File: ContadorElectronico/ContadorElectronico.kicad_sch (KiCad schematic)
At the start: 27 parts, among them J1 Screw_Terminal_01x02, J2 Screw_Terminal_01x02, SW1 MODE, SW2 INC, SW3 DEC, U4 LM358, U5 4N35, U6 4N35

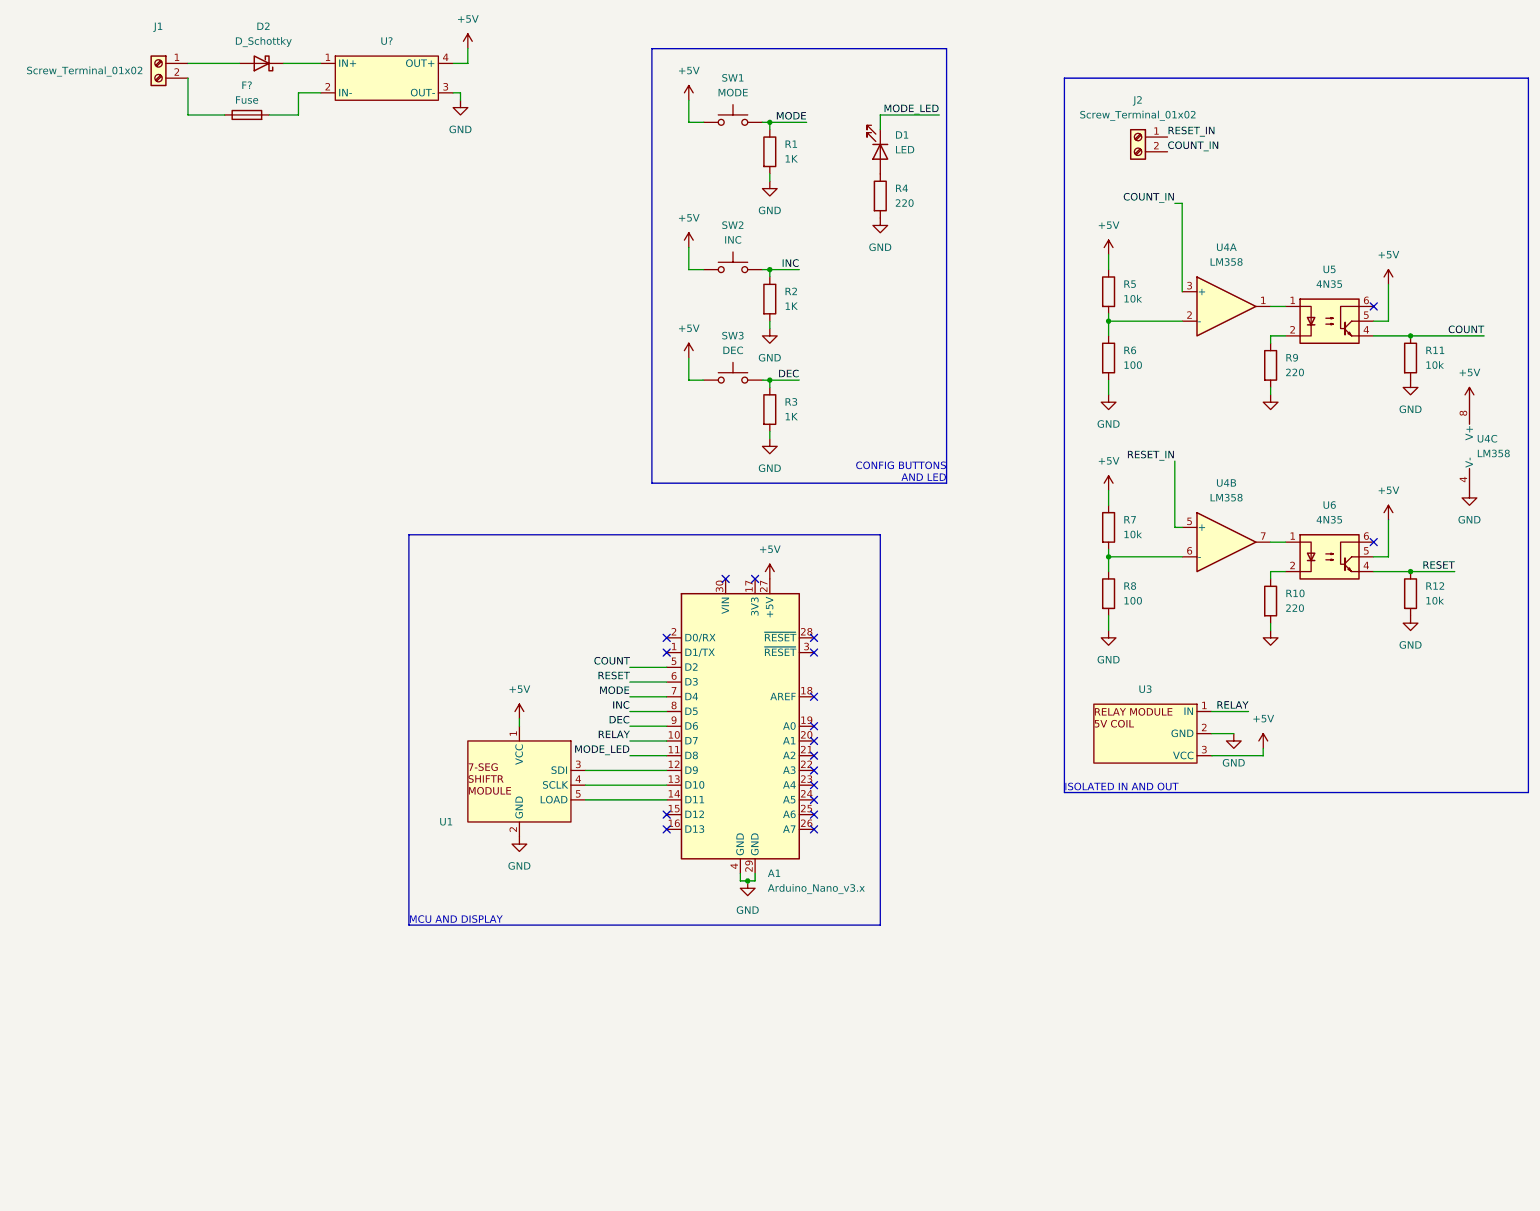
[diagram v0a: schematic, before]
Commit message: First PCB design
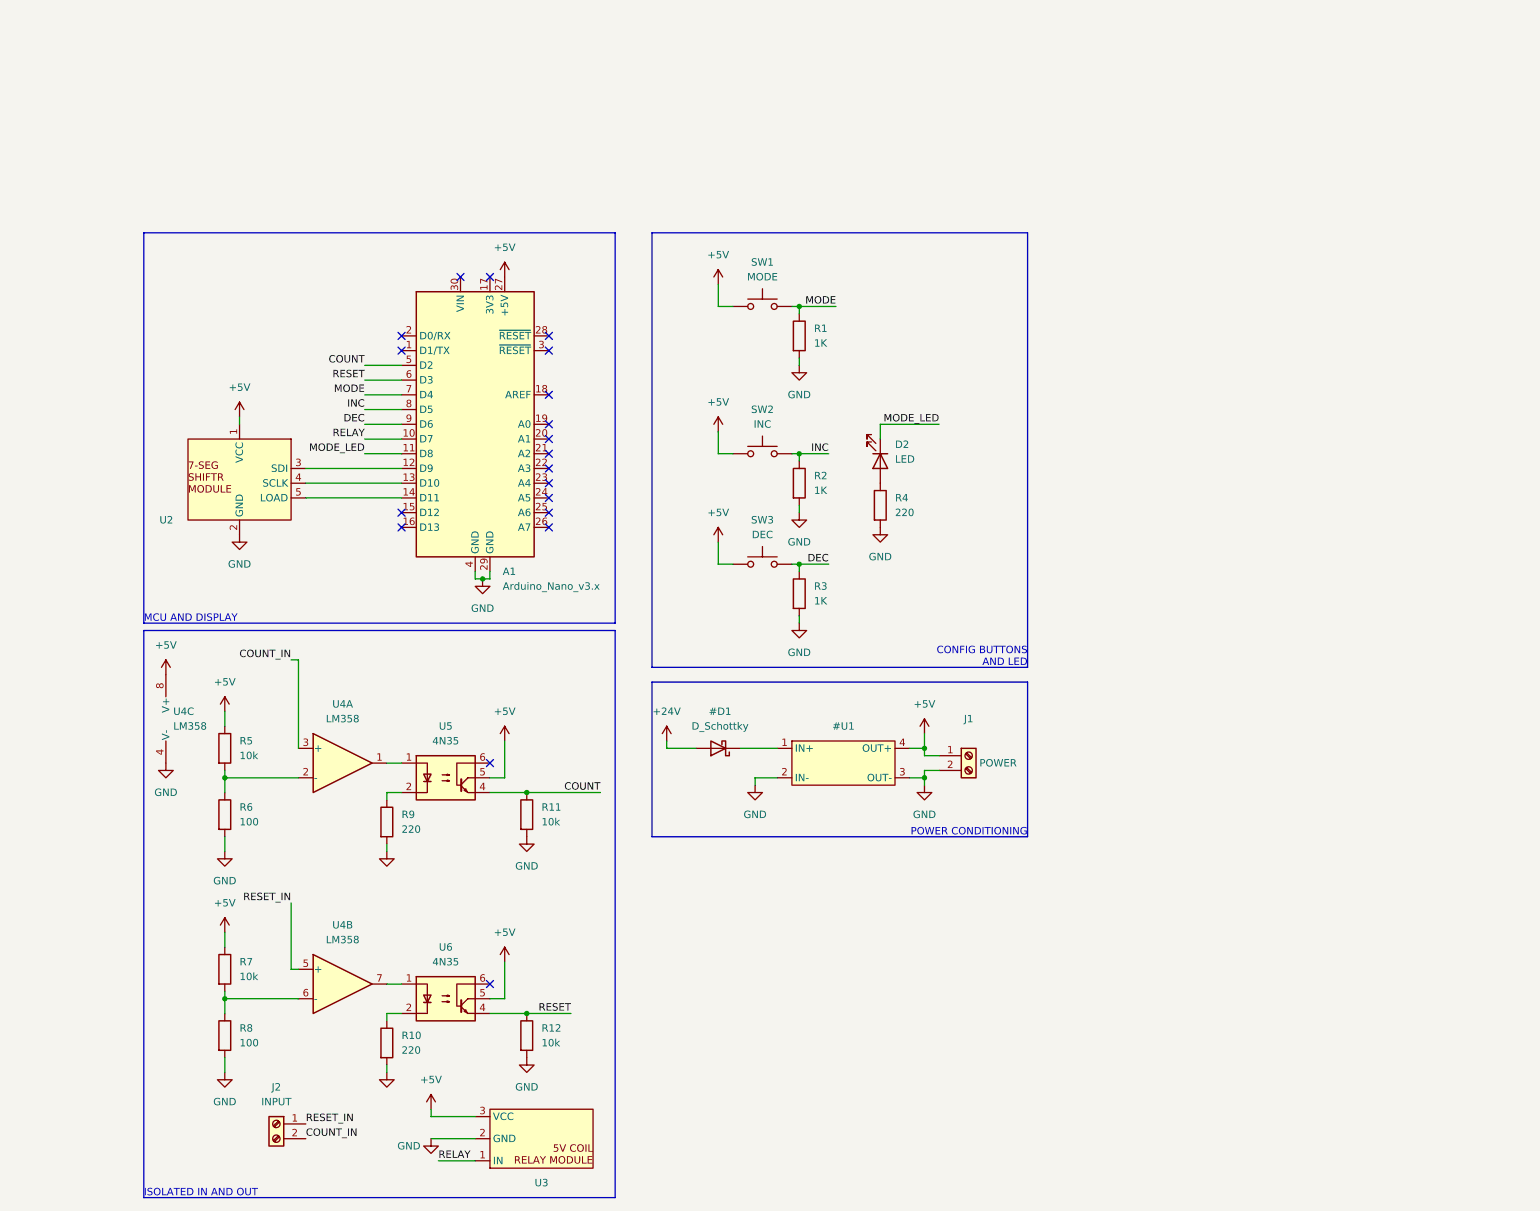
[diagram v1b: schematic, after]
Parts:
- removed F?: Fuse, symbol Device:Fuse
- J1: value Screw_Terminal_01x02 -> POWER
- J2: value Screw_Terminal_01x02 -> INPUT
- gave numbers to parts that had none: 1
- renumbered D2 to #D1, D1 to D2, U1 to U2
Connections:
- net +5V: now also J1.1 (Pin_1)
- net GND: now also #U1.2 (IN-), J1.2 (Pin_2)
- net +24V: now reaches #D1.2 (A)
- net +24V: no longer J1.1 (Pin_1)
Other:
- note added: "POWER CONDITIONING"
- moved on the sheet: A1, D2, J1, J2, R1, R10, R11, R12, R2, R3, R4, R5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
